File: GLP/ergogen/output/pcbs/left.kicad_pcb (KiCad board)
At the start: 2 copper layers, 138.8 x 106.7 mm, 65 parts

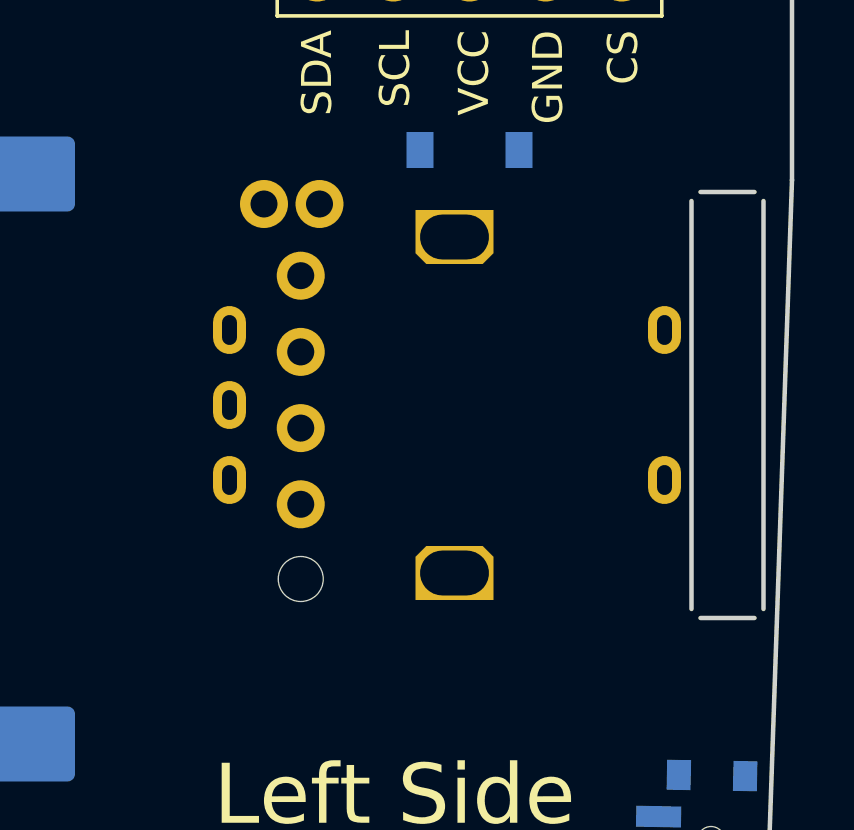
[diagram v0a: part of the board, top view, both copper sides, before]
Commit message: ok
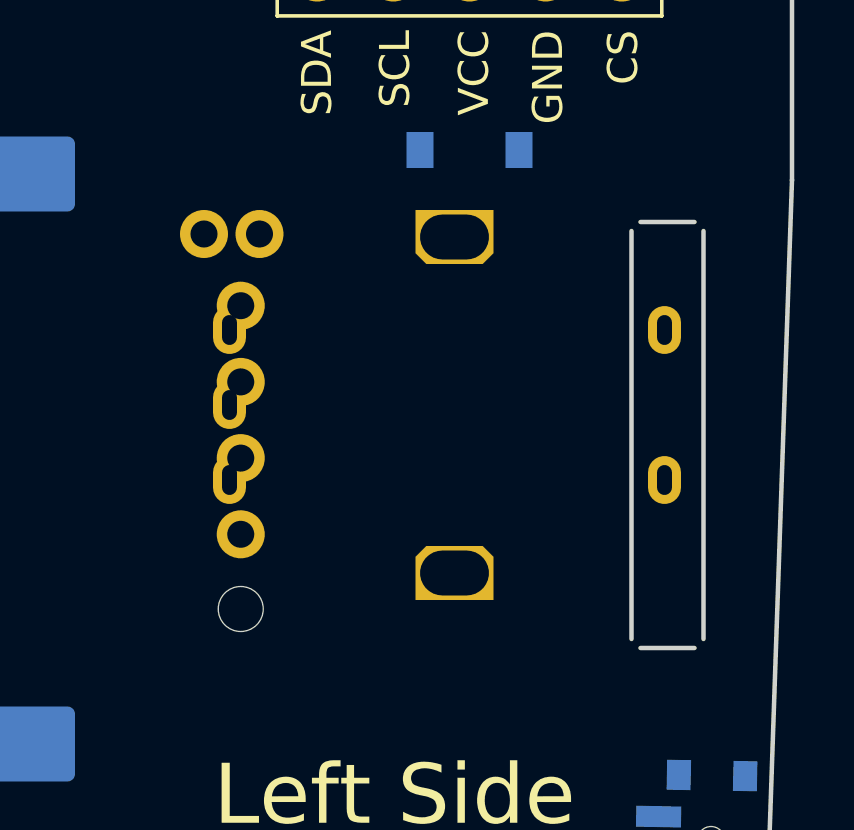
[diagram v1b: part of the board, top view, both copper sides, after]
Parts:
- moved REF** 2.24 mm to (165.5, 115.0)
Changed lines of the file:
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@@
   (title_block
     (title "left")
-    (date "2025-03-31")
+    (date "2025-04-01")
     (rev "v1.0.0")
     (company "Unknown")
@@
       (pad "2" smd rect (at 1.65 0 60) (size 0.9 1.2) (layers "B.Cu" "B.Paste" "B.Mask") (net 35 "space_cluster"))
     )
-      (module RollerEncoder_Panasonic_EVQWGD001 (layer F.Cu)
-      (at 167.5 114 0)
-      (fp_text reference REF** (at 0 0 0) (layer F.Fab) (effects (font (size 1 1) (thickness 0.15))))
-      (fp_text value RollerEncoder_Panasonic_EVQWGD001 (at -0.1 9 0) (layer F.Fab) (effects (font (size 1 1) (thickness 0.15))))
-      (fp_line (start -8.4 -6.4) (end 8.4 -6.4) (layer Dwgs.User) (width 0.12))
-      (fp_line (start 8.4 -6.4) (end 8.4 7.4) (layer Dwgs.User) (width 0.12))
-      (fp_line (start 8.4 7.4) (end -8.4 7.4) (layer Dwgs.User) (width 0.12))
-      (fp_line (start -8.4 7.4) (end -8.4 -6.4) (layer Dwgs.User) (width 0.12))
-        (fp_line (start 9.8 7.3) (end 9.8 -6.3) (layer Edge.Cuts) (width 0.15))
-        (fp_line (start 7.4 -6.3) (end 7.4 7.3) (layer Edge.Cuts) (width 0.15))
-        (fp_line (start 9.5 -6.6) (end 7.7 -6.6) (layer Edge.Cuts) (width 0.15))
-        (fp_line (start 7.7 7.6) (end 9.5 7.6) (layer Edge.Cuts) (width 0.15))
-        (pad S1 thru_hole circle (at -6.85 -6.2 0) (size 1.6 1.6) (drill 0.9) (layers *.Cu *.Mask) (net 27 "col5"))
-        (pad S2 thru_hole circle (at -5 -6.2 0) (size 1.6 1.6) (drill 0.9) (layers *.Cu *.Mask) (net 41 "scrollwheel_enc"))
-        (pad A thru_hole circle (at -5.625 -3.81 0) (size 1.6 1.6) (drill 0.9) (layers *.Cu *.Mask) (net 42 "ENCA"))
-        (pad B thru_hole circle (at -5.625 -1.27 0) (size 1.6 1.6) (drill 0.9) (layers *.Cu *.Mask) (net 3 "GND"))
-        (pad C thru_hole circle (at -5.625 1.27 0) (size 1.6 1.6) (drill 0.9) (layers *.Cu *.Mask) (net 42 "ENCA"))
-        (pad D thru_hole circle (at -5.625 3.81 0) (size 1.6 1.6) (drill 0.9) (layers *.Cu *.Mask) (net 43 "undef"))
-        (pad "" np_thru_hole circle (at -5.625 6.3 0) (size 1.5 1.5) (drill 1.5) (layers *.Cu *.Mask))
-      )
-    (footprint "ceoloide:diode_tht_sod123"
-        (layer "B.Cu")
+        (module RollerEncoder_Panasonic_EVQWGD001 (layer F.Cu)
+        (at 165.5 115 0)
+        (fp_text reference REF** (at 0 0 0) (layer F.Fab) (effects (font (size 1 1) (thickness 0.15))))
+        (fp_text value RollerEncoder_Panasonic_EVQWGD001 (at -0.1 9 0) (layer F.Fab) (effects (font (size 1 1) (thickness 0.15))))
+        (fp_line (start -8.4 -6.4) (end 8.4 -6.4) (layer Dwgs.User) (width 0.12))
+        (fp_line (start 8.4 -6.4) (end 8.4 7.4) (layer Dwgs.User) (width 0.12))
+        (fp_line (start 8.4 7.4) (end -8.4 7.4) (layer Dwgs.User) (width 0.12))
+        (fp_line (start -8.4 7.4) (end -8.4 -6.4) (layer Dwgs.User) (width 0.12))
+          (fp_line (start 9.8 7.3) (end 9.8 -6.3) (layer Edge.Cuts) (width 0.15))
+          (fp_line (start 7.4 -6.3) (end 7.4 7.3) (layer Edge.Cuts) (width 0.15))
+          (fp_line (start 9.5 -6.6) (end 7.7 -6.6) (layer Edge.Cuts) (width 0.15))
+          (fp_line (start 7.7 7.6) (end 9.5 7.6) (layer Edge.Cuts) (width 0.15))
+          (pad S1 thru_hole circle (at -6.85 -6.2 0) (size 1.6 1.6) (drill 0.9) (layers *.Cu *.Mask) (net 27 "col5"))
+          (pad S2 thru_hole circle (at -5 -6.2 0) (size 1.6 1.6) (drill 0.9) (layers *.Cu *.Mask) (net 41 "scrollwheel_enc"))
+          (pad A thru_hole circle (at -5.625 -3.81 0) (size 1.6 1.6) (drill 0.9) (layers *.Cu *.Mask) (net 42 "ENCA"))
+          (pad B thru_hole circle (at -5.625 -1.27 0) (size 1.6 1.6) (drill 0.9) (layers *.Cu *.Mask) (net 3 "GND"))
+          (pad C thru_hole circle (at -5.625 1.27 0) (size 1.6 1.6) (drill 0.9) (layers *.Cu *.Mask) (net 42 "ENCA"))
+          (pad D thru_hole circle (at -5.625 3.81 0) (size 1.6 1.6) (drill 0.9) (layers *.Cu *.Mask) (net 43 "undef"))
+          (pad "" np_thru_hole circle (at -5.625 6.3 0) (size 1.5 1.5) (drill 1.5) (layers *.Cu *.Mask))
+        )
+    (footprint "ceoloide:diode_tht_sod123"
+        (layer "B.Cu")

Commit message: almost finsihed ergogen config for glp
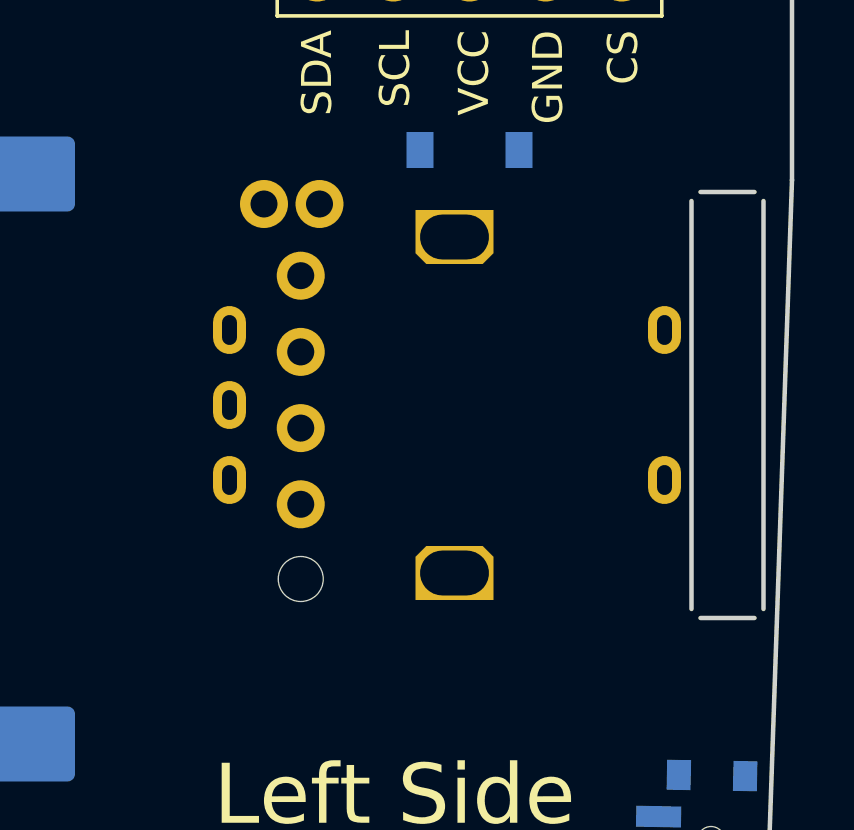
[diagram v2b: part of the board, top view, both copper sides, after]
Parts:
- moved REF** 2.24 mm to (167.5, 114.0)
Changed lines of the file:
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@@
     )
         (module RollerEncoder_Panasonic_EVQWGD001 (layer F.Cu)
-        (at 165.5 115 0)
+        (at 167.5 114 0)
         (fp_text reference REF** (at 0 0 0) (layer F.Fab) (effects (font (size 1 1) (thickness 0.15))))
         (fp_text value RollerEncoder_Panasonic_EVQWGD001 (at -0.1 9 0) (layer F.Fab) (effects (font (size 1 1) (thickness 0.15))))
